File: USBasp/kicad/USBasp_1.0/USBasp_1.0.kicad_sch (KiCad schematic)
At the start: 11 parts, among them J1 USB_B, U1 ATmega8-16PU, Y1 12MHz

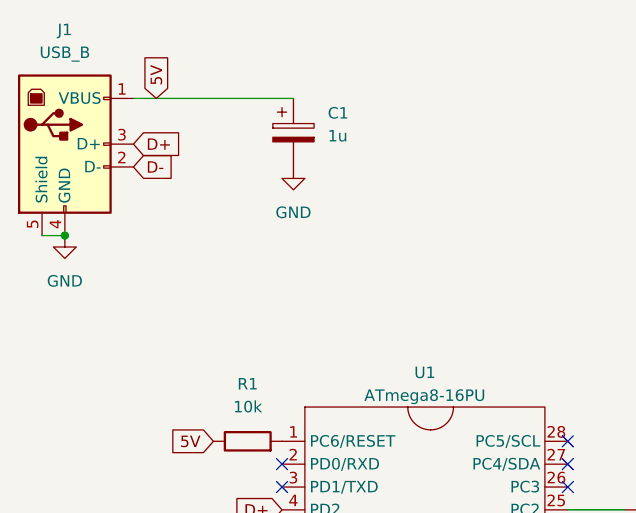
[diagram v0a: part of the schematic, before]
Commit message: update
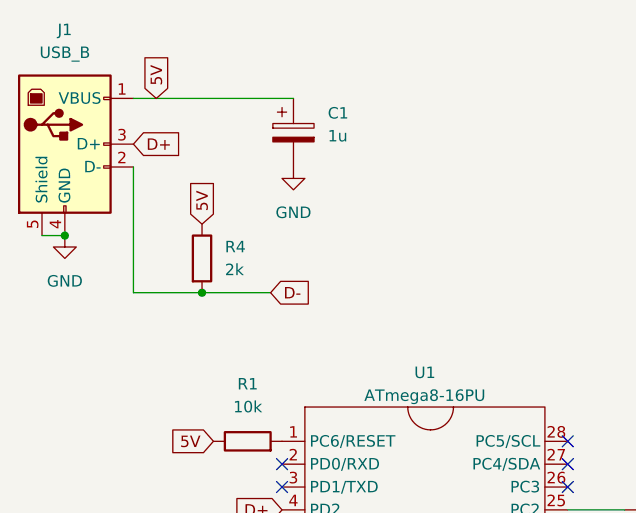
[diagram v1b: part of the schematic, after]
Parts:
- added R4: 2k, symbol Device:R
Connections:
- net 5V: now also R4.1
- net D-: now also R4.2
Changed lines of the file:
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@@
+	)
+	(junction
+		(at 41.91 48.26)
+		(diameter 0)
+		(color 0 0 0 0)
 	)
 	(junction
@@
 	(wire
 		(pts
+			(xy 34.29 48.26) (xy 34.29 34.29)
+		)
+		(stroke
+			(width 0)
+			(type default)
+		)
+	)
+	(wire
+		(pts
 			(xy 24.13 41.91) (xy 26.67 41.91)
 		)
@@
 	(wire
 		(pts
+			(xy 41.91 48.26) (xy 34.29 48.26)
+		)
+		(stroke
+			(width 0)
+			(type default)
+		)
+	)
+	(wire
+		(pts
 			(xy 38.1 133.35) (xy 40.64 133.35)
 		)
@@
 		(pts
 			(xy 36.83 82.55) (xy 50.8 82.55)
+		)
+		(stroke
+			(width 0)
+			(type default)
+		)
+	)
+	(wire
+		(pts
+			(xy 49.53 48.26) (xy 41.91 48.26)
 		)
 		(stroke
@@
 	(global_label "D-"
 		(shape input)
-		(at 34.29 34.29 0)
+		(at 49.53 48.26 0)
 		(fields_autoplaced yes)
 		(effects
@@
 		)
 		(property "Intersheetrefs" "${INTERSHEET_REFS}"
-			(at 40.1176 34.29 0)
+			(at 55.3576 48.26 0)
 			(effects
 				(font
@@
 		(property "Intersheetrefs" "${INTERSHEET_REFS}"
 			(at 40.1176 31.75 0)
+			(effects
+				(font
+					(size 1.27 1.27)
+				)
+				(justify left)
+				(hide yes)
+			)
+		)
+	)
+	(global_label "5V"
+		(shape input)
+		(at 41.91 40.64 90)
+		(fields_autoplaced yes)
+		(effects
+			(font
+				(size 1.27 1.27)
+			)
+			(justify left)
+		)
+		(property "Intersheetrefs" "${INTERSHEET_REFS}"
+			(at 41.91 35.3567 90)
 			(effects
 				(font
@@
 					(unit 1)
 				)
+			)
+		)
+	)
+	(symbol
+		(lib_id "Device:R")
+		(at 41.91 44.45 0)
+		(unit 1)
+		(exclude_from_sim no)
+		(in_bom yes)
+		(on_board yes)
+		(dnp no)
+		(fields_autoplaced yes)
+		(property "Reference" "R4"
+			(at 44.45 43.1799 0)
+			(effects
+				(font
+					(size 1.27 1.27)
+				)
+				(justify left)
+			)
+		)
+		(property "Value" "2k"
+			(at 44.45 45.7199 0)
+			(effects
+				(font
+					(size 1.27 1.27)
+				)
+				(justify left)
+			)
+		)
+		(property "Footprint" ""
+			(at 40.132 44.45 90)
+			(effects
+				(font
+					(size 1.27 1.27)
+				)
+				(hide yes)
+			)
+		)
+		(property "Datasheet" "~"
+			(at 41.91 44.45 0)
+			(effects
+				(font
+					(size 1.27 1.27)
+				)
+				(hide yes)
+			)
+		)
+		(property "Description" "Resistor"
+			(at 41.91 44.45 0)
+			(effects
+				(font
+					(size 1.27 1.27)
+				)
+				(hide yes)
+			)
+		)
+		(pin "1"
+		)
+		(pin "2"
+		)
+		(instances
+			(project "USBasp_1.0"
+				(path "/3d8db78b-f3e8-43dd-b475-5cbf51decb09"
+					(reference "R4")
+					(unit 1)
+				)
